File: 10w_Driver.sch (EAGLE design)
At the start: 35 parts, among them IC1 78L05Z, IC2 WS2811-SOP8, T1 2N3904, T2 2N3904, T3 2N3904, U1 PT4115PT4115B89E, U2 PT4115PT4115B89E, U3 PT4115PT4115B89E, X1 22-23-2031, X2 22-23-2031, X3 LED-PAD, X4 LED-PAD, X5 LED-PAD, X6 LED-PAD, X7 LED-PAD, X8 LED-PAD

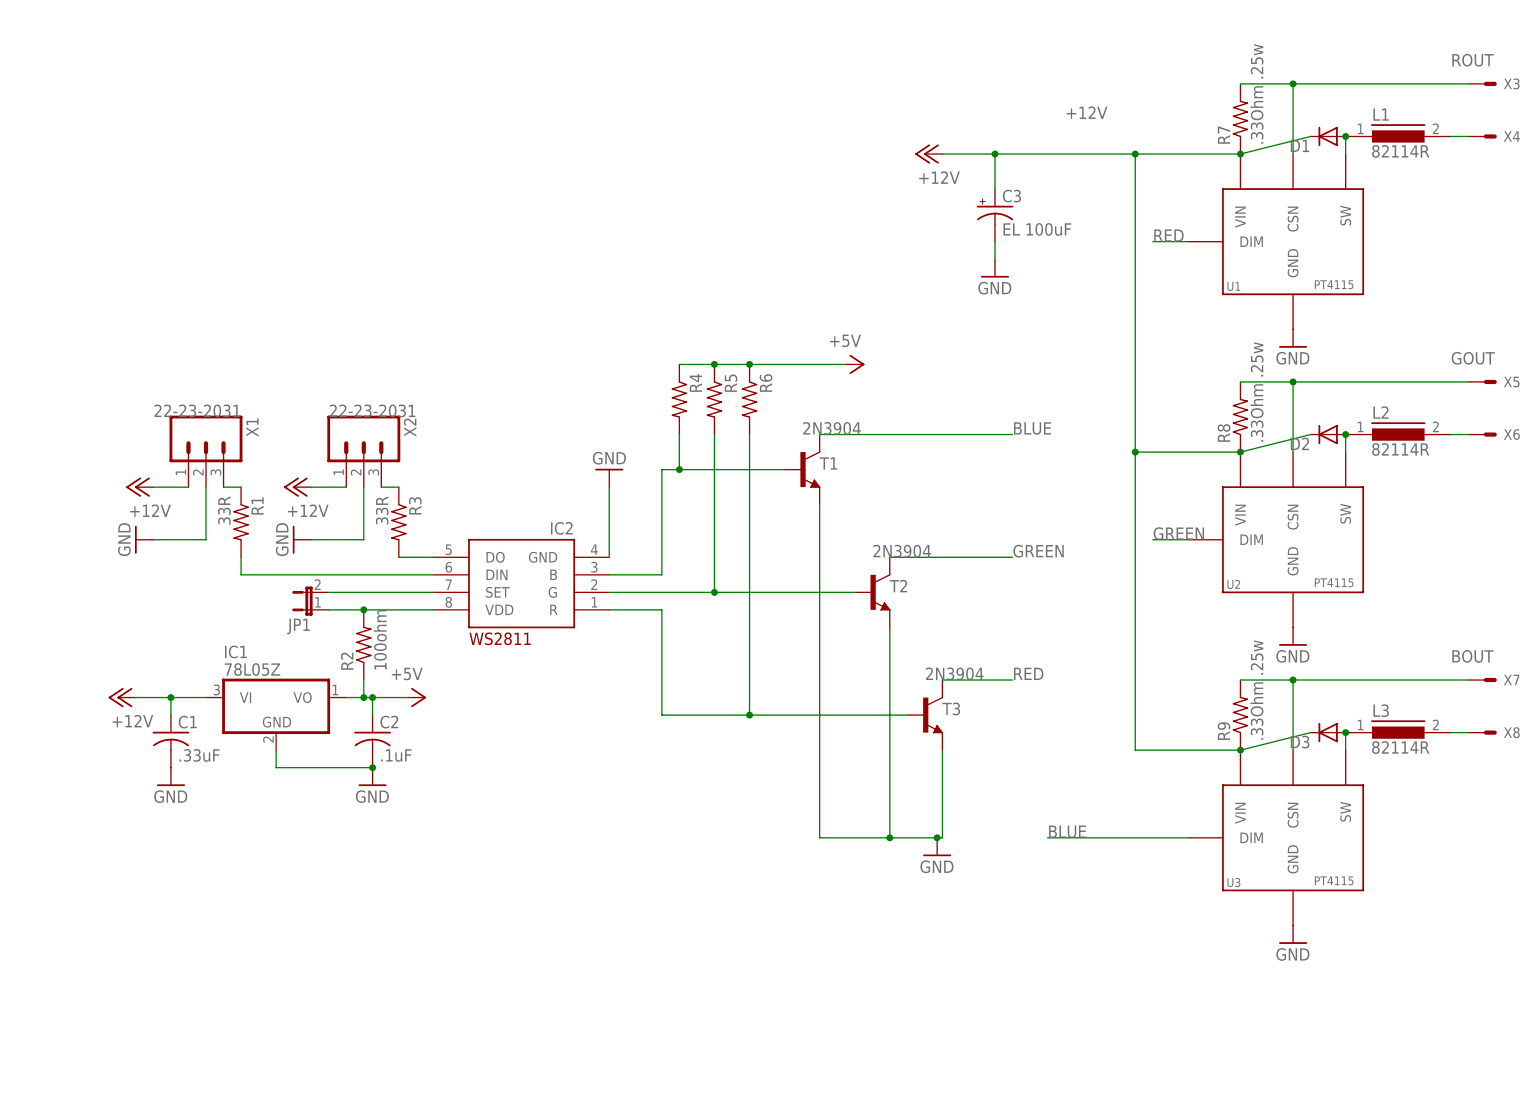
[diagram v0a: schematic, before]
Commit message: Reworked Layout
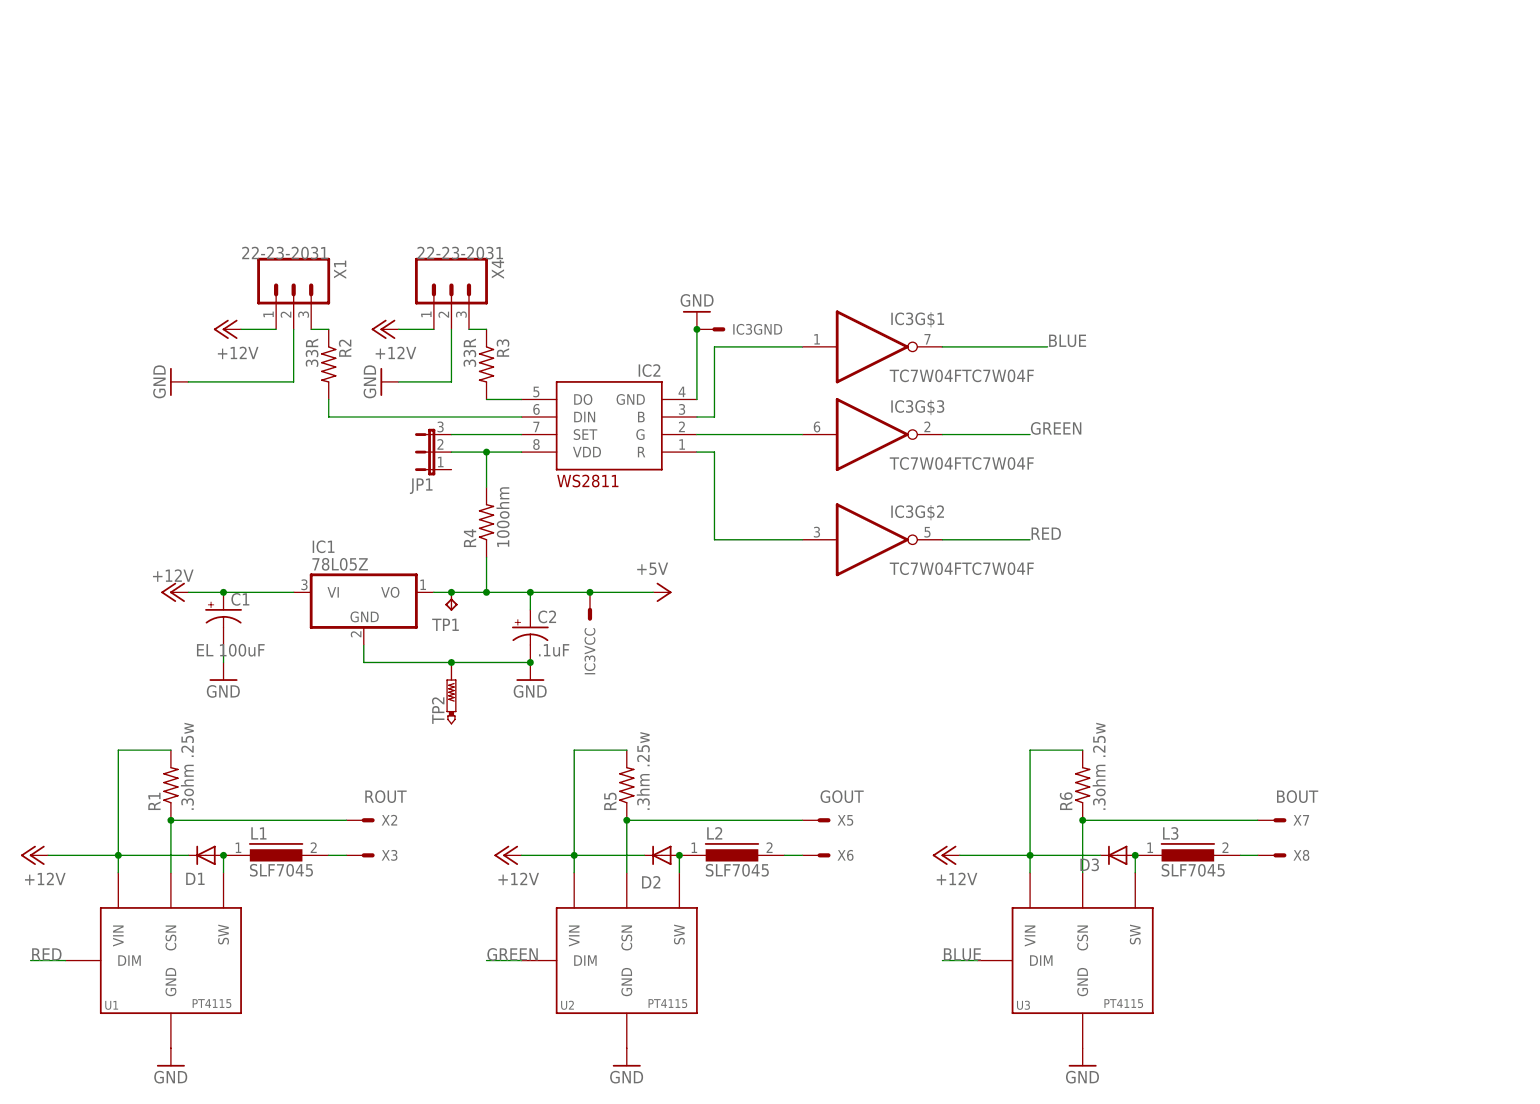
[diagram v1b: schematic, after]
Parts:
- removed C3: EL 100uF, rcl:CPOL-USTT2D6L
- removed R7, R8, R9: .33Ohm .25w, resistor:R-US_0204/5
- removed T1, T2, T3: 2N3904, transistor:2N3904
- added IC3: TC7W04FTC7W04F, MyLibrary:TC7W04FTC7W04F
- added TP1: TPB2,54, testpad:TPB2,54
- added TP2: PTR1TP20SQ, testpad:PTR1TP20SQ
- C1: value .33uF -> EL 100uF; device rcl:C-US025-025X050 -> rcl:CPOL-USTT2D6L
- C2: device rcl:C-US025-025X050 -> resistor:CPOL-USB45181A
- JP1: device jumper:JP1E -> jumper:JP2E
- L1, L2, L3: value 82114R -> SLF7045; device inductors:82114R -> inductors:SLF7045
- R1: value 33R -> .3ohm .25w; device rcl:R-US_0204/5 -> resistor:R-US_R1206
- R2: value 100ohm -> 33R; device rcl:R-US_0204/5 -> rcl:R-US_M0805
- R3: device rcl:R-US_0204/5 -> rcl:R-US_M0805
- R4: value (none) -> 100ohm; device resistor:R-US_0204/5 -> rcl:R-US_M0805
- R5: value (none) -> .3hm .25w; device resistor:R-US_0204/5 -> resistor:R-US_M1206
- R6: value (none) -> .3ohm .25w; device resistor:R-US_0204/5 -> resistor:R-US_R1206
- U1, U2, U3: device MyLibrary:PT4115PT4115B89E -> IC:PT4115PT4115B89E
- X2: value 22-23-2031 -> LED-PAD; device MyLibrary:22-23-2031 -> MyLibrary:LED-PAD
- X4: value LED-PAD -> 22-23-2031; device MyLibrary:LED-PAD -> MyLibrary:22-23-2031
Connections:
- removed net N$20: IC2.R, R6.2, T3.B
- new net N$19: IC2.G, IC3G$3.I
- net +12V: now also C1.+, R1.2, R5.2, R6.2, X4.1; no longer C1.1, C3.+, R7.1, R8.1, R9.1, X2.1
- net +5V: now also C2.+, IC3VCC.S, TP1.TP; no longer C2.1, R2.1, R5.1, R6.1
- net BLUE: now also IC3G$1.O; no longer T1.C
- net BOUT: now also R6.1; no longer R9.2
- net GND: now also C1.-, C2.-, IC3GND.S, TP2.TP, X4.2; no longer C1.2, C2.2, C3.-, T1.E, T2.E, T3.E, X2.2
- net GOUT: now also R5.1; no longer R8.2
- net GREEN: now also IC3G$3.O; no longer T2.C
- net N$14: now also JP1.2, R4.2; no longer JP1.1, R2.2
- net N$15: now also IC2.R, IC3G$2.I; no longer IC2.B, R4.2, T1.B
- net N$16: now also IC2.B, IC3G$1.I; no longer IC2.SET, JP1.2
- net N$18: now also IC2.SET, JP1.3; no longer IC2.G, R5.2, T2.B
- net N$3: now also X3.S; no longer X4.S
- net N$4: now also X4.3; no longer X2.3
- net N$6: now also R2.1; no longer R1.1
- net N$8: now also R2.2; no longer R1.2
- net RED: now also IC3G$2.O; no longer T3.C
- net ROUT: now also R1.1, X2.S; no longer R7.2, X3.S
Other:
- moved on the sheet: D1, D2, D3, IC1, IC2, R1, R2, R3, R4, R5, R6, U1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
